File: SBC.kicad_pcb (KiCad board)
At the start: 2 copper layers, 160 x 100.3 mm, 97 parts, among them K1 A17, K10 BNKSEL, K11 16K/32K, K12 INTSEL, K13 RSTSEL, K6 A18, K7 128/512, K8 A19, K9 PWR, P1 IDE, P2 POWER, P3 SERIAL, P4 CLK_CPU, P5 CLK_UART, P6 RESET, Q1 2N3906, SW1 RESETSW, U1 16550, U10 74LS243, U11 74LS245, U12 74LS174, U13 74LS174, U14 74LS32, U15 74LS32, U16 74LS32, U17 74LS244, U18 74LS174, U19 8255, U2 27C080, U20 C96ABC, U21 DS1302, U22 MAX232, U23 SRAM_512KO, U24 Z80-CPU, U25 DS1210, U26 74LS06N, U27 74LS14, U3 74LS08, U4 74LS10, U5 74LS125, U6 74LS139, U7 74LS14, U8 74LS245, U9 74LS245, X1 CRYSTAL

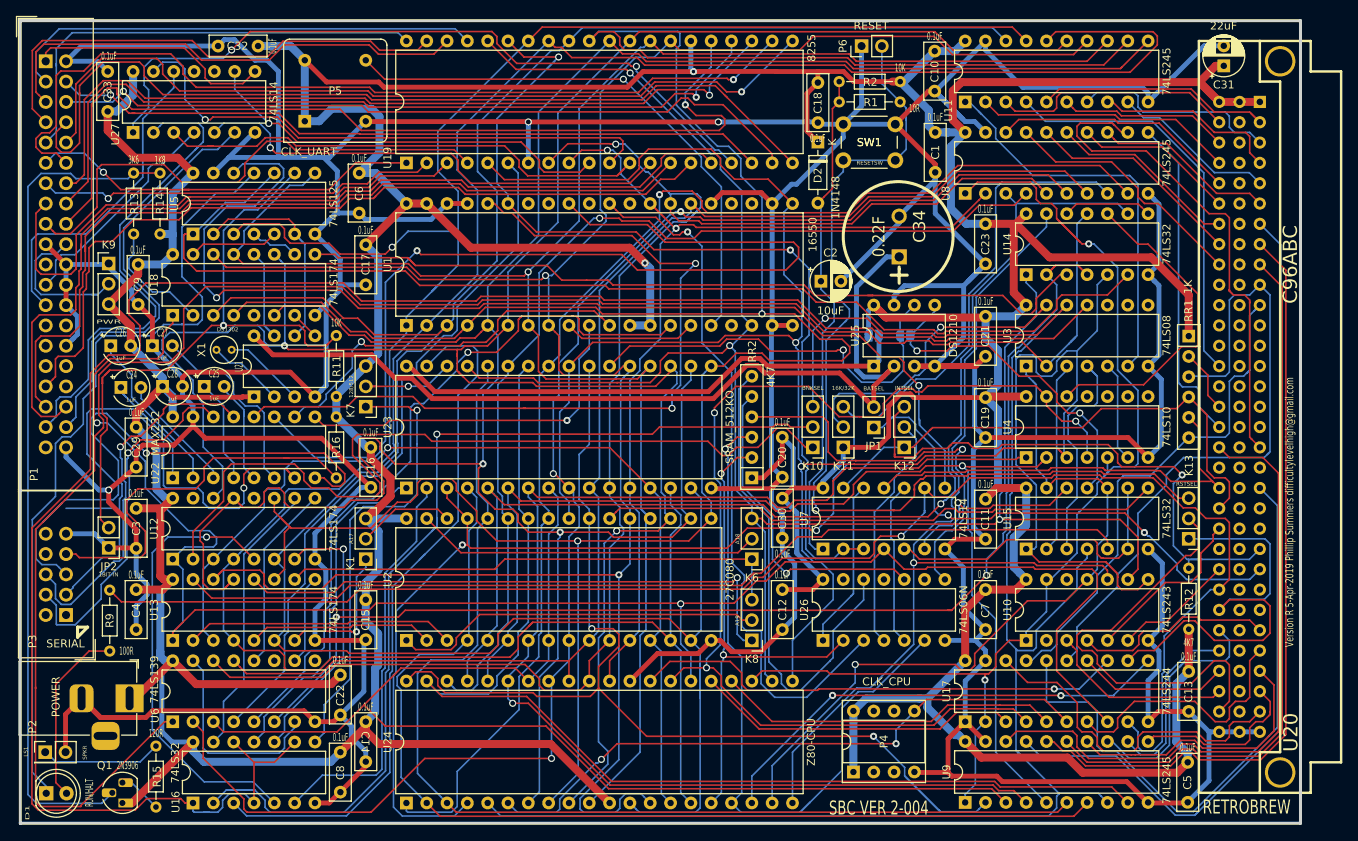
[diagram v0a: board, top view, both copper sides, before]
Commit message: Version S
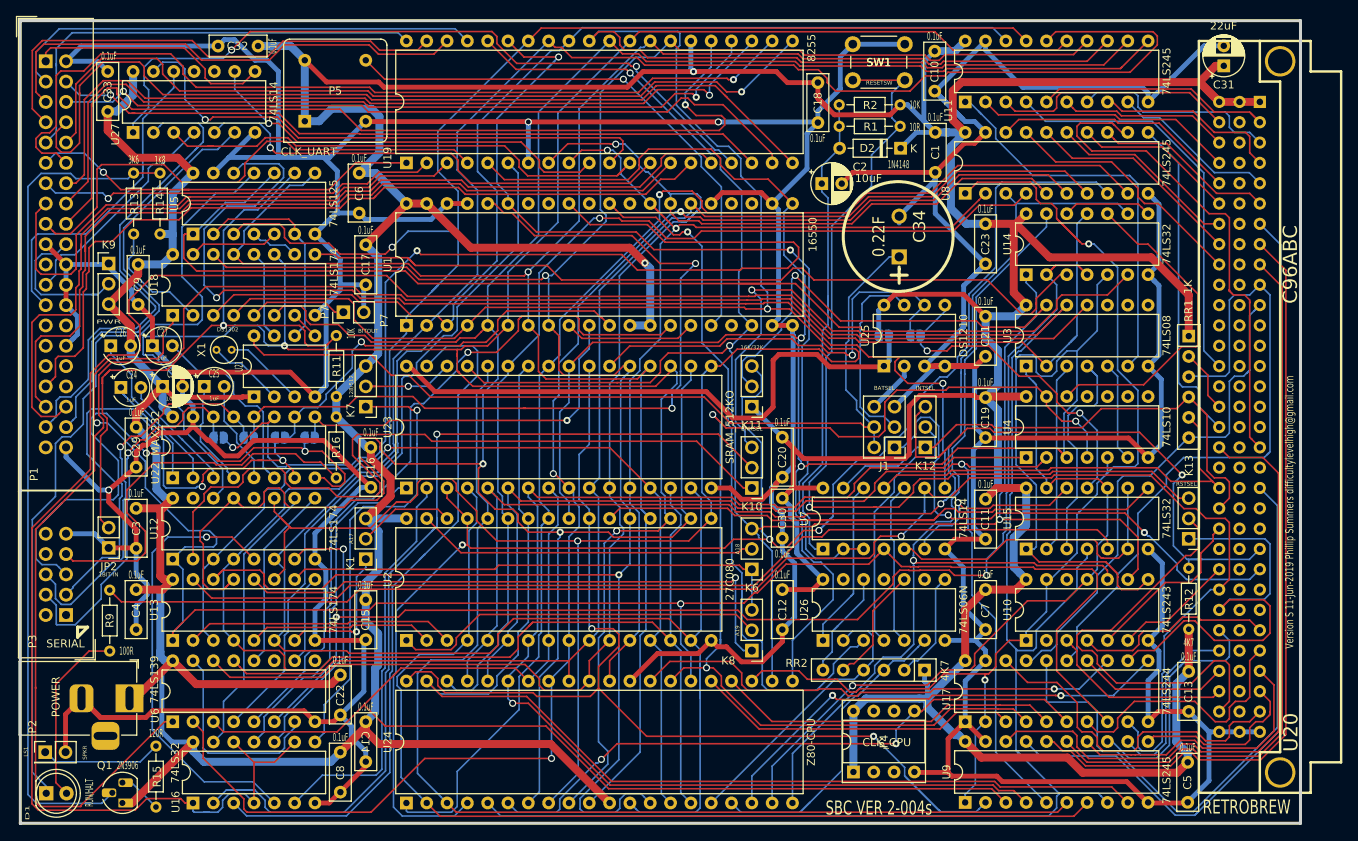
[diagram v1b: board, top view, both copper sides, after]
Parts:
- removed JP1: BATSEL, Connector_PinHeader_2.54mm:PinHeader_1x02_P2.54mm_Vertical
- removed P6: RESET, Connector_PinHeader_2.54mm:PinHeader_1x02_P2.54mm_Vertical
- added G***: LOGO, phil.summers:SOLDERBRIDGES, B.Cu at (150.0, 143.5)
- added G***: LOGO, phil.summers:JUMPERSET3, B.Cu at (144.8, 123.5)
- added G***: LOGO, phil.summers:JUMPERSET2, B.Cu at (144.7, 104.1)
- added G***: LOGO, phil.summers:EPROM JUMPERS, B.Cu at (149.7, 63.6)
- added J1: BATSEL, Connector_PinHeader_2.54mm:PinHeader_2x03_P2.54mm_Vertical, F.Cu at (186.7, 106.7)
- added JP5: RXD, Jumper:SolderJumper-2_P1.3mm_Open_RoundedPad1.0x1.5mm, B.Cu at (113.6, 105.5)
- added JP6: CTS, Jumper:SolderJumper-2_P1.3mm_Open_RoundedPad1.0x1.5mm, B.Cu at (106.0, 105.5)
- added JP7: TXD, Jumper:SolderJumper-2_P1.3mm_Open_RoundedPad1.0x1.5mm, B.Cu at (109.9, 105.5)
- added JP8: RTS, Jumper:SolderJumper-2_P1.3mm_Open_RoundedPad1.0x1.5mm, B.Cu at (102.3, 105.5)
- added P7: BITOUT, Connector_PinHeader_2.54mm:PinHeader_1x02_P2.54mm_Vertical, F.Cu at (117.9, 89.8)
- C28: value 1uF -> 10uF; footprint Capacitor_THT:CP_Radial_Tantal_D4.5mm_P2.50mm -> Capacitor_THT:CP_Radial_D5.0mm_P2.50mm
- moved RR2 32.3 mm to (190.5, 134.5), turned to 180 degrees
- moved K11 12.5 mm to (168.9, 101.6)
- moved C2 12.2 mm to (177.6, 73.7)
- moved D2 10.4 mm to (187.5, 69.3), turned to 180 degrees
- moved SW1 10.1 mm to (181.5, 56.3)
- moved K10 9.16 mm to (168.9, 111.8)
- moved R1 3.05 mm to (179.8, 66.5)
- moved R2 2.90 mm to (187.5, 63.9)
- moved K12 2.64 mm to (190.6, 106.7)
- moved JP4 1.27 mm to (189.4, 92.7)
- moved K8 1.27 mm to (168.9, 132.1)
- moved K6 1.27 mm to (168.9, 121.9)
- moved JP3 1.27 mm to (185.4, 92.7)
- moved U25 1.27 mm to (185.4, 96.5)
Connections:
- net /NC_A23 renamed /~B_IQ0
- C34 pad 1: /VBAT1 -> Net-(C34-Pad1)
- RR2 pad 2: //INT -> /PU1K-A
- RR2 pad 4: /PU1K-A -> //INT
- U21 pad 8: /VBAT1 -> Net-(C34-Pad1)
- U25 pad 7: GND -> /VBAT2
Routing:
- net Net-(C34-Pad1): track 0.00 -> 111.8 mm
- net /VBAT1: track 114.8 -> 6.64 mm
- net //NMI: track 89.3 -> 39.6 mm, vias 1 -> 0
- net /PU1K-C: track 61.2 -> 14.2 mm
- net /PU1K-A: track 50.9 -> 13.8 mm, vias 1 -> 0
- net //INT: track 62.6 -> 35.1 mm, vias 2 -> 0
- net /A14: track 173.0 -> 199.3 mm, vias 2 -> 3
- net /PU1K-B: track 40.3 -> 14.8 mm, vias 1 -> 0
- net /VBAT2: track 0.00 -> 24.5 mm
- net /A15: track 211.9 -> 232.9 mm
- net //CS_ROM: track 70.7 -> 87.6 mm
- net Net-(K11-Pad2): track 39.9 -> 55.2 mm
- net /RTS_TTL: track 124.2 -> 137.7 mm, vias 1 -> 2
- net Net-(P7-Pad1): track 0.00 -> 12.4 mm
- net VCC: track 935.7 -> 926.9 mm
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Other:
- board text added: "SBC VER 2-004s"
- board text added: "Version S 11-Jun-2019 Phillip Summers difficultylevelhigh@gmail.com"
- board text removed: "SBC VER 2-004"
- board text removed: "Version R 5-Apr-2019 Phillip Summers difficultylevelhigh@gmail.com"

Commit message: Version T
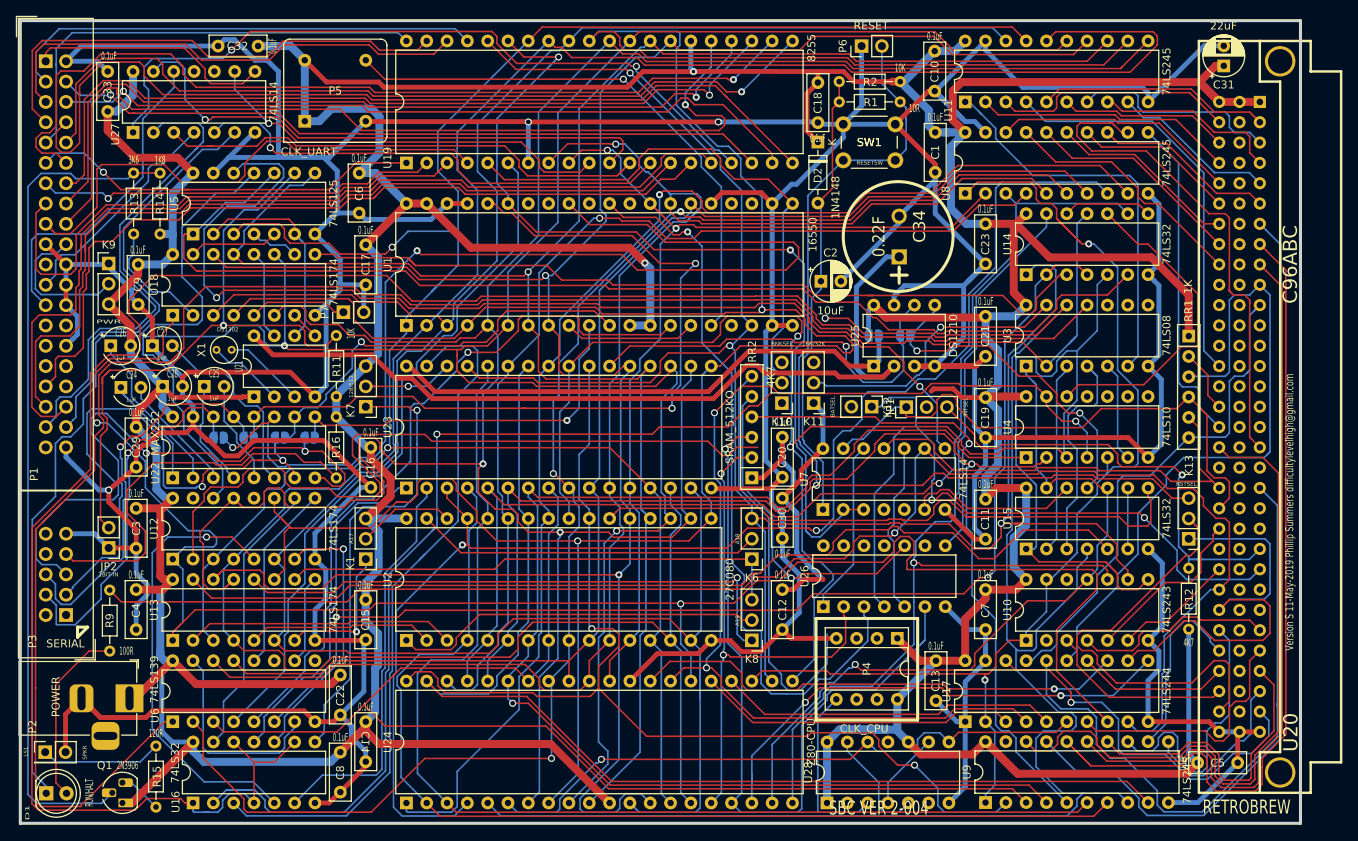
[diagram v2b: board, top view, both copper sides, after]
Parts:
- removed G***: LOGO, phil.summers:SOLDERBRIDGES
- removed G***: LOGO, phil.summers:JUMPERSET3
- removed G***: LOGO, phil.summers:JUMPERSET2
- removed G***: LOGO, phil.summers:EPROM JUMPERS
- removed J1: BATSEL, Connector_PinHeader_2.54mm:PinHeader_2x03_P2.54mm_Vertical
- added JP1: BATSEL, Connector_PinHeader_2.54mm:PinHeader_1x02_P2.54mm_Vertical, F.Cu at (183.9, 101.6)
- added P6: RESET, Connector_PinHeader_2.54mm:PinHeader_1x02_P2.54mm_Vertical, F.Cu at (182.6, 56.5)
- added U28: 74LS74, Package_DIP:DIP-14_W7.62mm, F.Cu at (178.3, 151.1)
- C28: value 10uF -> 1uF; footprint Capacitor_THT:CP_Radial_D5.0mm_P2.50mm -> Capacitor_THT:CP_Radial_Tantal_D4.5mm_P2.50mm
- moved RR2 32.3 mm to (168.9, 110.5), turned to 90 degrees
- moved C13 31.6 mm to (191.9, 133.3)
- moved P4 17.6 mm to (187.1, 130.6), turned to 270 degrees
- moved C2 12.2 mm to (177.5, 85.9)
- moved K10 11.3 mm to (172.7, 101.1)
- moved D2 10.4 mm to (177.2, 68.5), turned to 270 degrees
- moved SW1 10.1 mm to (180.3, 66.3)
- moved K11 7.74 mm to (176.6, 101.1)
- moved K12 5.57 mm to (188.2, 101.7), turned to 90 degrees
- moved U7 4.93 mm to (177.8, 114.5)
- moved U26 4.22 mm to (177.9, 126.6)
- moved R1 3.05 mm to (179.8, 63.5)
- moved R2 2.90 mm to (187.5, 61.0)
- moved U9 2.54 mm to (198.1, 151.1)
- moved JP4 1.27 mm to (188.1, 92.7)
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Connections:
- net /~B_IQ0 renamed /NC_A23
- net Net-(P7-Pad1) renamed /TURBO
- C34 pad 1: Net-(C34-Pad1) -> /VBAT1
- P4 pad 5: /CLK_CPU -> Net-(P4-Pad5)
- RR2 pad 2: /PU1K-A -> //INT
- RR2 pad 4: //INT -> /PU1K-A
- U21 pad 8: Net-(C34-Pad1) -> /VBAT1
- U25 pad 7: /VBAT2 -> GND
- U26 pad 12: /PU1K-C -> Net-(U26-Pad12)
- U26 pad 13: Net-(U26-Pad13) -> Net-(P4-Pad5)
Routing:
- net Net-(C34-Pad1): track 111.8 -> 0.00 mm
- net /VBAT1: track 6.64 -> 110.0 mm
- net //NMI: track 39.6 -> 94.5 mm, vias 0 -> 1
- net /PU1K-C: track 14.2 -> 52.5 mm
- net //INT: track 35.1 -> 67.4 mm, vias 0 -> 2
- net Net-(U15-Pad6): track 39.3 -> 7.62 mm
- net /PU1K-A: track 13.8 -> 42.9 mm, vias 0 -> 1
- net /A14: track 199.3 -> 172.4 mm, vias 3 -> 2
- net /PU1K-B: track 14.8 -> 41.6 mm, vias 0 -> 1
- net /VBAT2: track 24.5 -> 0.00 mm
- net Net-(P4-Pad5): track 0.00 -> 21.7 mm
- net /A15: track 232.9 -> 211.5 mm
- net Net-(K11-Pad2): track 55.2 -> 37.9 mm
- net GND: track 948.2 -> 932.1 mm
- net //RD: track 282.9 -> 298.0 mm
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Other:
- board text added: "SBC VER 2-004"
- board text added: "Version S 11-May-2019 Phillip Summers difficultylevelhigh@gmail.com"
- board text removed: "SBC VER 2-004s"
- board text removed: "Version S 11-Jun-2019 Phillip Summers difficultylevelhigh@gmail.com"
